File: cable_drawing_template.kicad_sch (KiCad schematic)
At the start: 3 parts

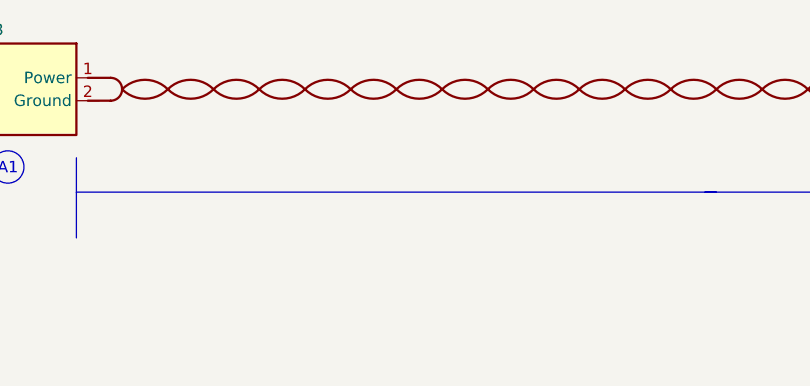
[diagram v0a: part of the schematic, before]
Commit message: preliminary final
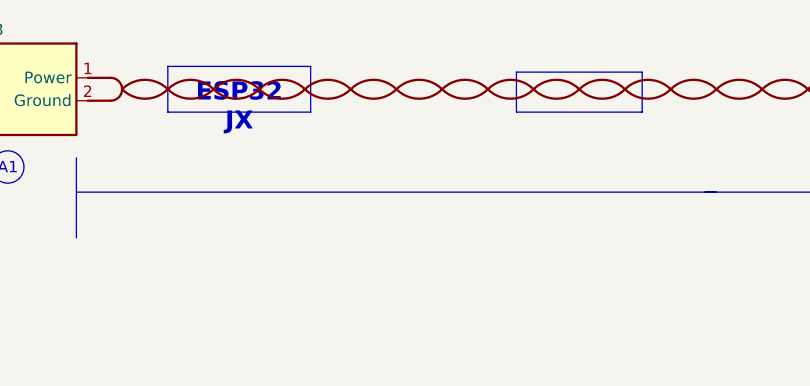
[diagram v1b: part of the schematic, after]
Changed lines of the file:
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@@
+		)
+	)
+	(rectangle
+		(start 113.665 94.615)
+		(end 127.635 99.06)
+		(stroke
+			(width 0)
+			(type default)
+		)
+		(fill
+			(type color)
+			(color 255 255 194 1)
 		)
 	)
@@
 		)
 	)
+	(text_box "ESP32 JX"
+		(exclude_from_sim no)
+		(at 74.93 93.98 0)
+		(size 15.875 5.08)
+		(stroke
+			(width 0)
+			(type default)
+		)
+		(fill
+			(type color)
+			(color 255 255 194 1)
+		)
+		(effects
+			(font
+				(size 2 2)
+				(thickness 0.4)
+				(bold yes)
+			)
+			(justify top)
+		)
+	)
